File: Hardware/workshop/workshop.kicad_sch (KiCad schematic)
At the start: 1 part, among them U101 NE555D

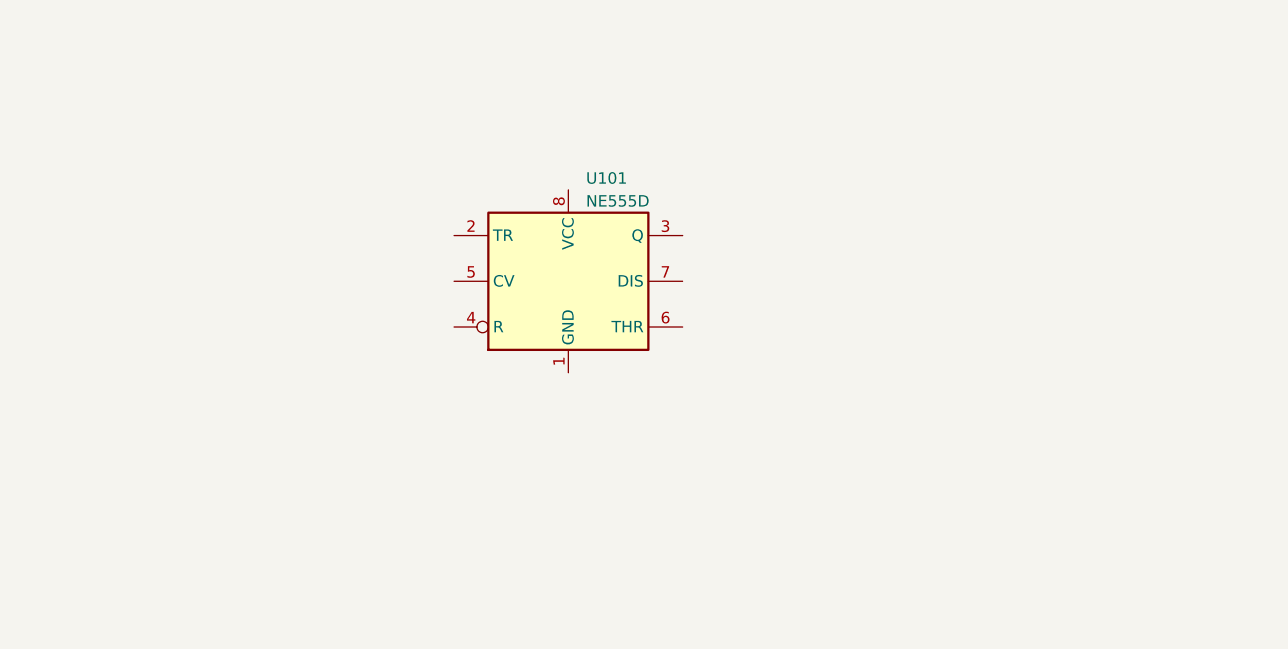
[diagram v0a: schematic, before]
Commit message: pcb workshop pcb
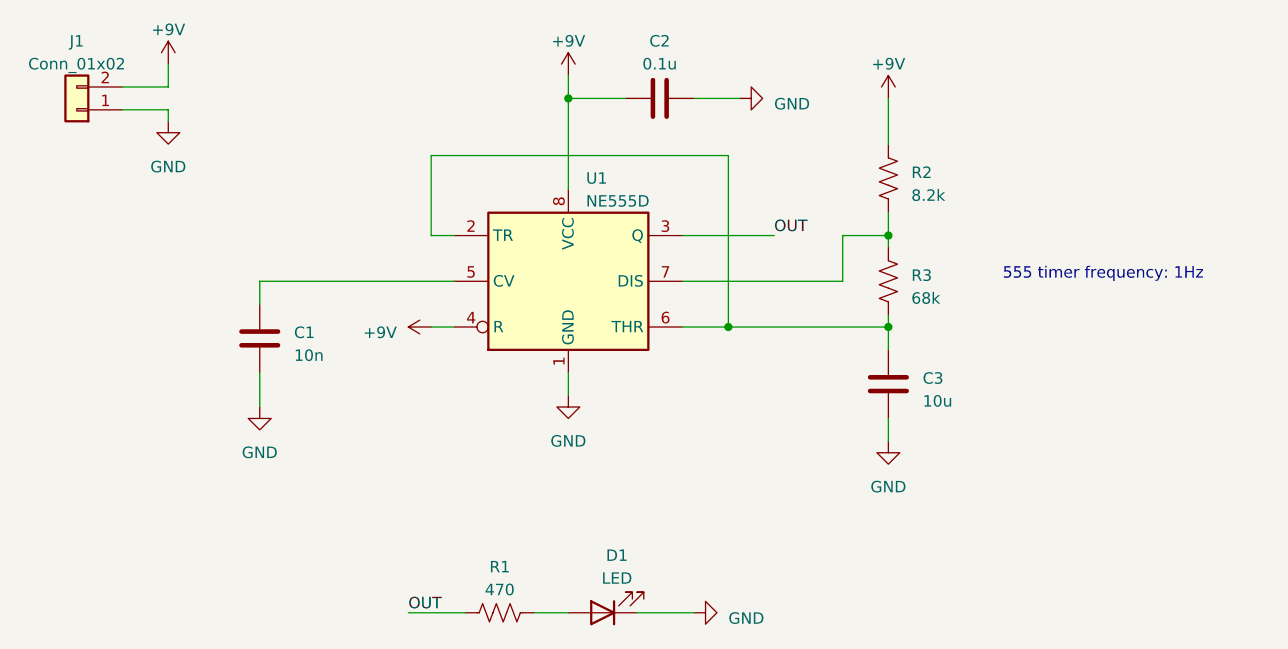
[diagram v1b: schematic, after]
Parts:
- added C1: 10n, Capacitor_SMD:C_0805_2012Metric, symbol Device:C
- added C2: 0.1u, Capacitor_SMD:C_0805_2012Metric, symbol Device:C
- added C3: 10u, Capacitor_SMD:C_0805_2012Metric, symbol Device:C
- added D1: LED, LED_THT:LED_D3.0mm, symbol Device:LED
- added J1: Conn_01x02, Connector_JST:JST_XH_B2B-XH-A_1x02_P2.50mm_Vertical, symbol Connector_Generic:Conn_01x02
- added R1: 470, Resistor_SMD:R_0805_2012Metric, symbol Device:R_US
- added R2: 8.2k, Resistor_SMD:R_0805_2012Metric, symbol Device:R_US
- added R3: 68k, Resistor_SMD:R_0805_2012Metric, symbol Device:R_US
- renumbered U101 to U1
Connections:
- net GND: now reaches U1.1 (GND)
- net GND: now also C1.1, C2.2, C3.1, D1.1 (K), J1.1 (Pin_1)
- net at U1.2 (TR): now also U1.6 (THR), C3.2, R3.2
- net OUT: now reaches U1.3 (Q)
- net OUT: now also R1.1
- net +9V: now reaches U1.4 (R)
- net +9V: now also U1.8 (VCC), C2.1, J1.2 (Pin_2), R2.1
- net at U1.5 (CV): now also C1.2
- net at U1.7 (DIS): now also R2.2, R3.1
- new net: D1.2 (A), R1.2
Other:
- note added: "555 timer frequency: 1Hz"
